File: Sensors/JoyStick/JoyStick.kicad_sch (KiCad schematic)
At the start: 55 parts, among them J1 USB_C_Receptacle_USB2.0_14P, J2 Conn_01x02, SW1 SW_SPST, U1 CR2013-MI2120, U2 ESP32-WROOM-32, U3 CH340C, U4 AMS1117-3.3, U5 LM386, U6 TP4056-42-ESOP8, X1 SW_Push, Y1 SW_Push

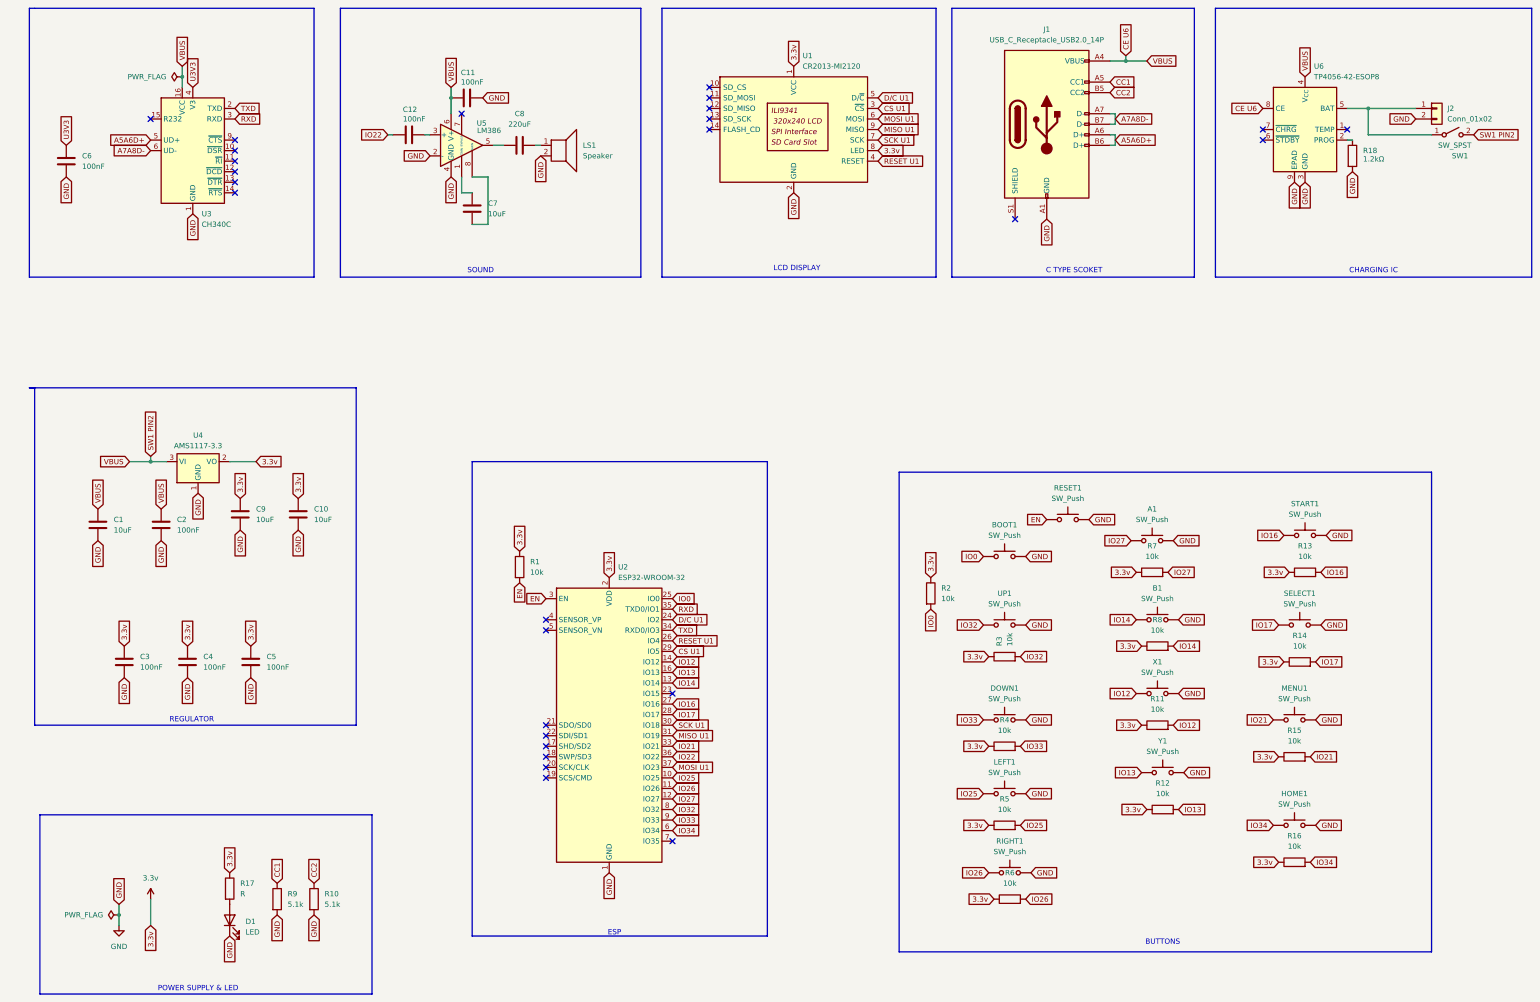
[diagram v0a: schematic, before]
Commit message: Initial Commit
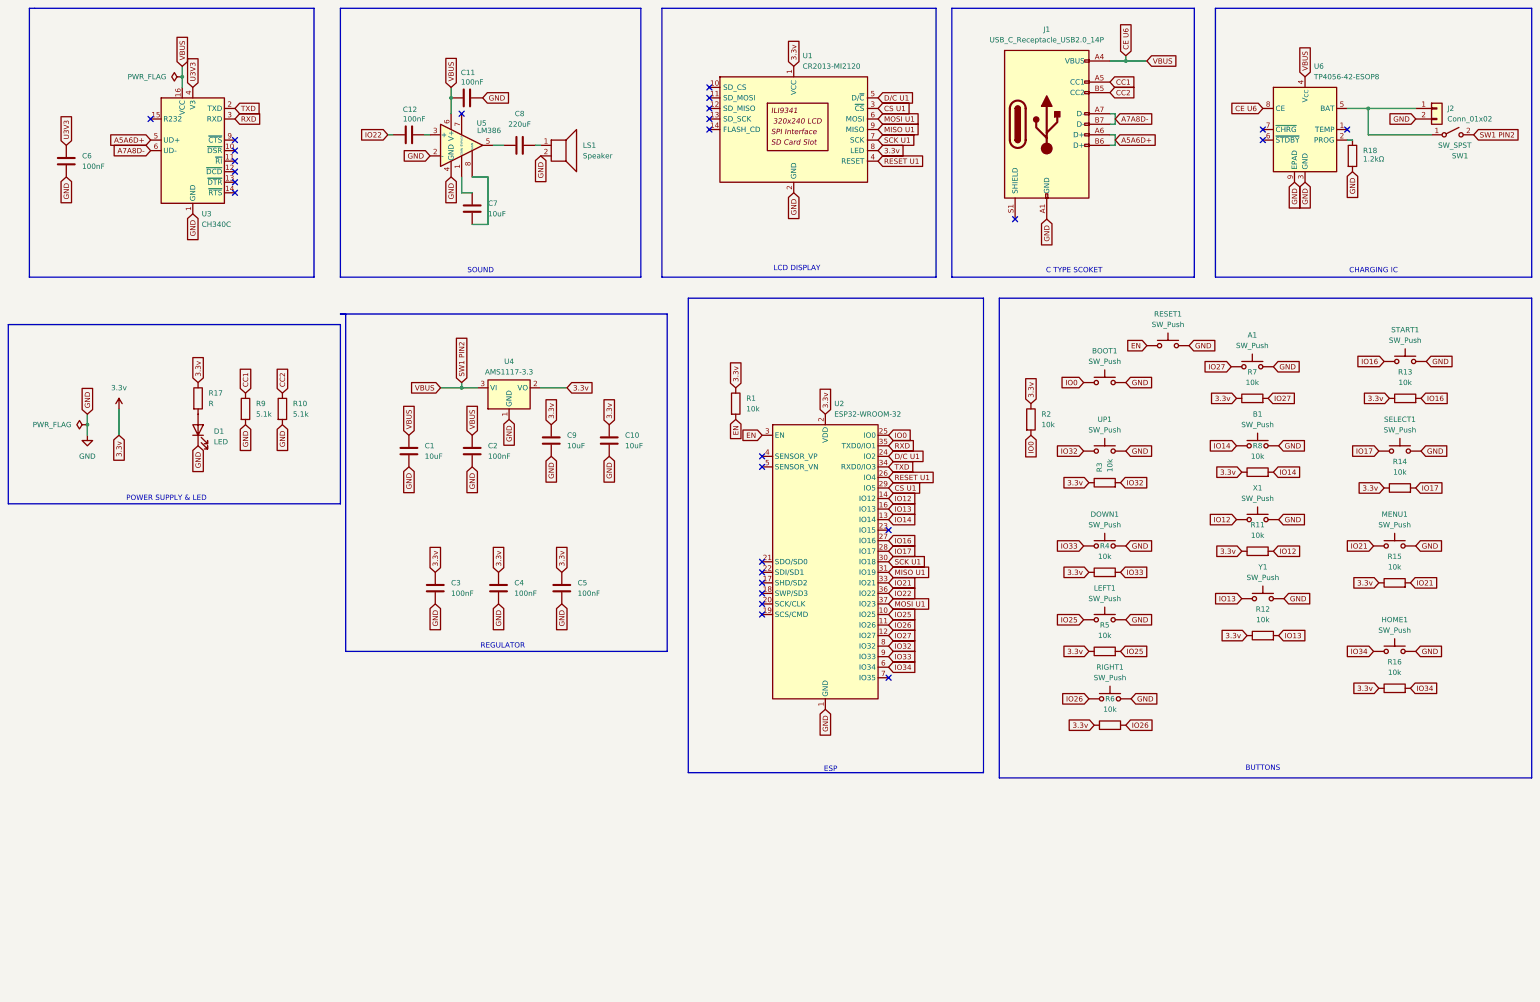
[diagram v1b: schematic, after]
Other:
- moved on the sheet: A1, B1, BOOT1, C1, C10, C2, C3, C4, C5, C9, D1, DOWN1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
